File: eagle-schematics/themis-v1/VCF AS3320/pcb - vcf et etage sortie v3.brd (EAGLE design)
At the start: 83.1 x 64.8 mm, 41 parts

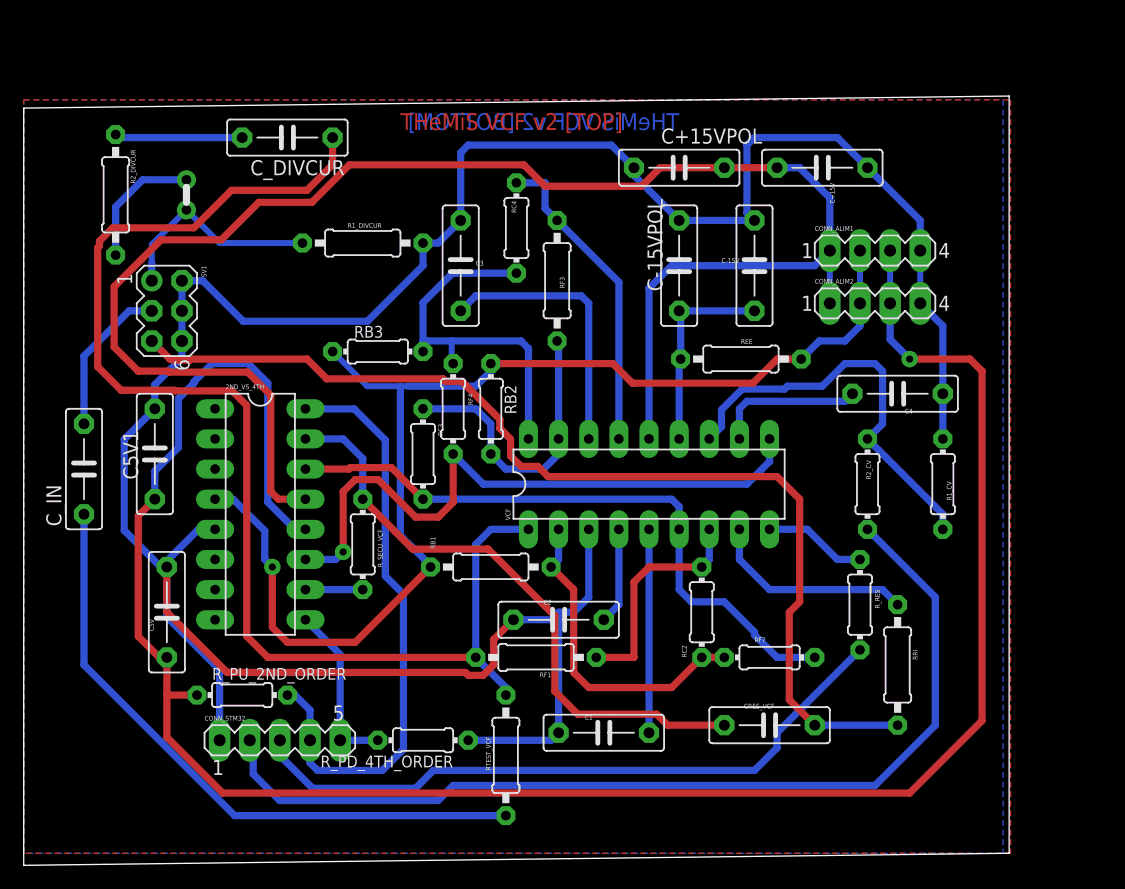
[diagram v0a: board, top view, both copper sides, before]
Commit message: schematic fix
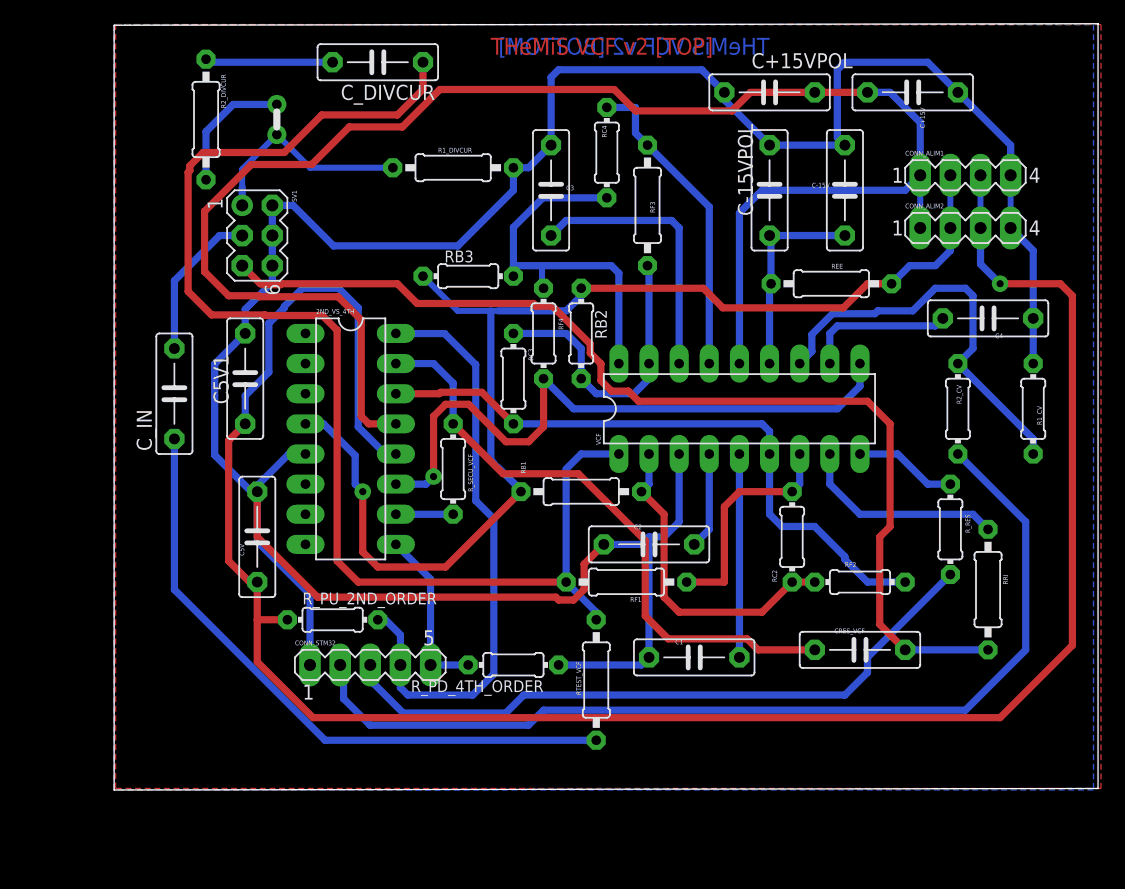
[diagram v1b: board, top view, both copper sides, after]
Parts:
- moved C+15V 9.92 mm to (67.3, 59.1)
- moved RC4 9.92 mm to (41.5, 54.0)
- moved RF2 9.92 mm to (62.9, 17.8)
- moved C1 9.92 mm to (48.9, 11.4)
- moved CRES_VCF 9.92 mm to (62.9, 12.1)
- moved C_DIVCUR 9.92 mm to (22.2, 61.6)
- moved R1_CV 9.92 mm to (77.5, 32.4)
- moved R1_DIVCUR 9.92 mm to (28.6, 52.7)
- moved R2_CV 9.92 mm to (71.1, 32.4)
- moved RF4 9.92 mm to (36.2, 38.7)
- moved R_SECU_VCF 9.92 mm to (28.6, 27.3)
- moved C5V 9.92 mm to (12.1, 21.6)
- moved CONN_STM32 9.92 mm to (21.6, 10.8)
- moved C_IN 9.92 mm to (5.08, 33.7)
- moved JP_MIXER_OUT 9.92 mm to (13.7, 56.8)
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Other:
- board size 83.1 x 64.8 mm -> 82.9 x 64.6 mm
